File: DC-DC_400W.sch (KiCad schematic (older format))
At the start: 12 parts, among them J1 Conn_01x24, J2 Conn_01x03, J3 Conn_01x10, J4 Conn_01x10, J5 Conn_01x01, J6 Conn_01x02, J7 Conn_01x01, J8 Conn_01x01, J9 Conn_01x01

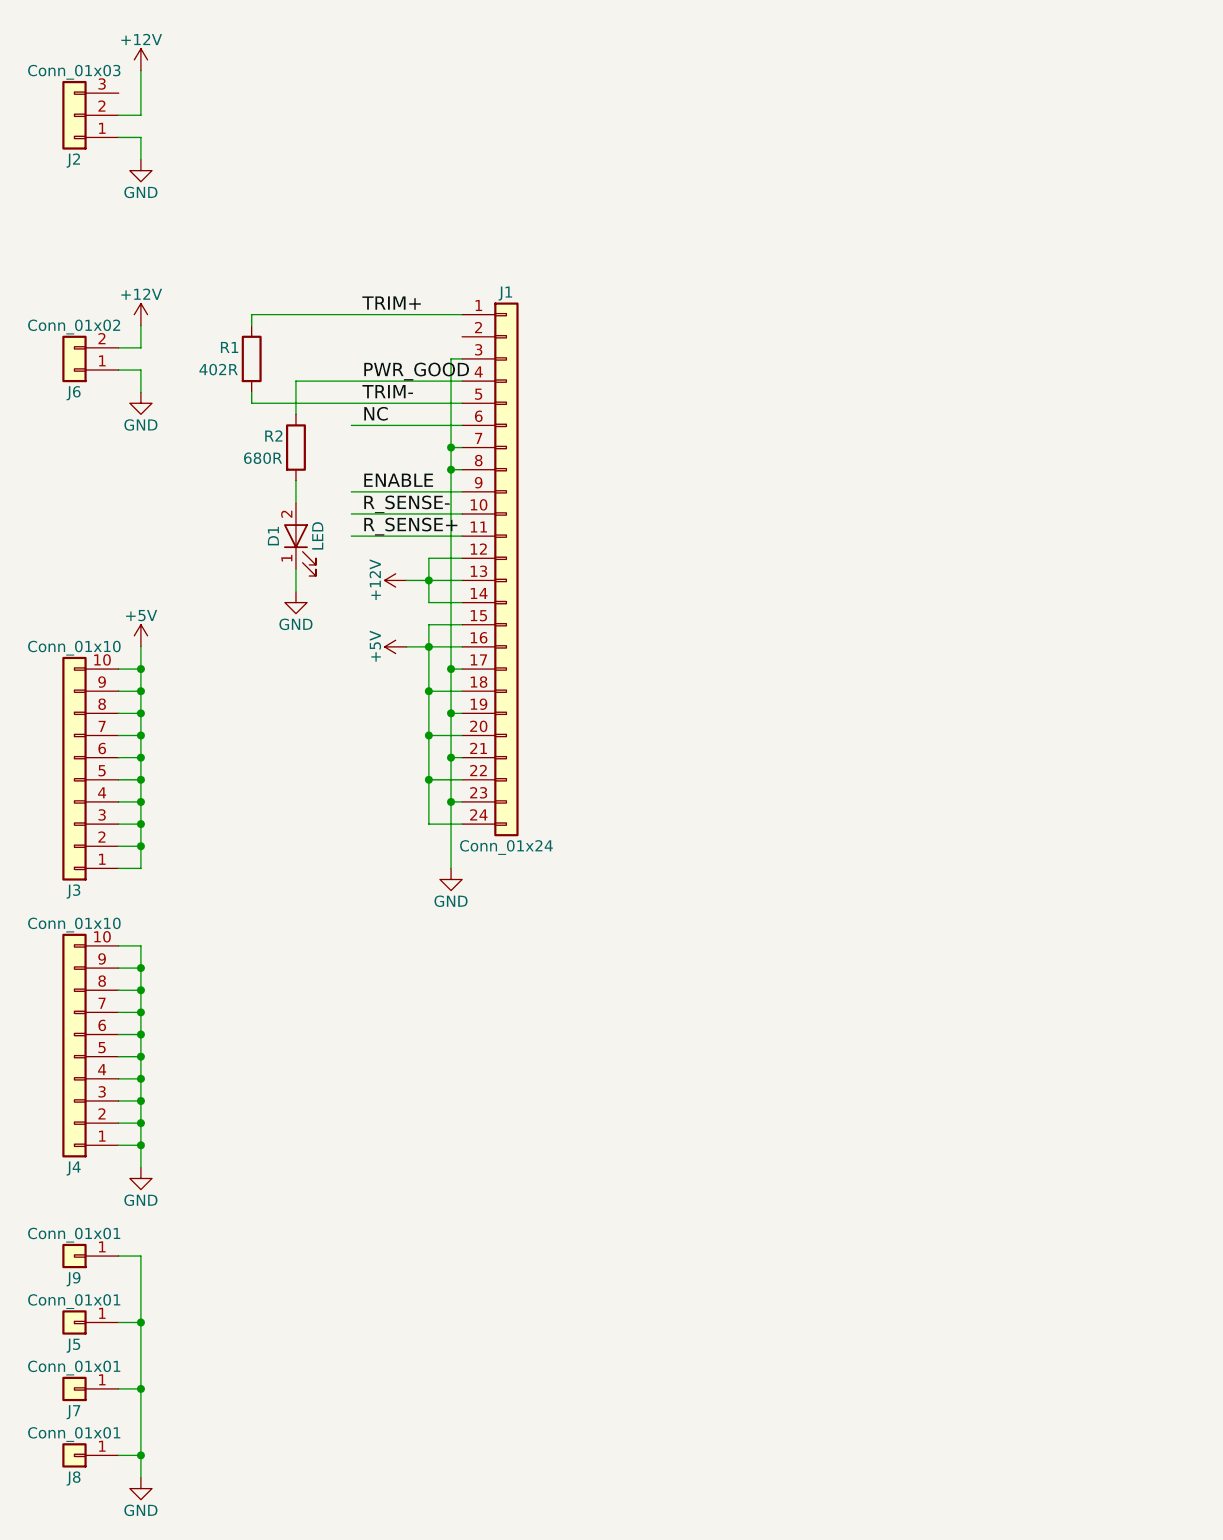
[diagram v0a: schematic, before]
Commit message: almost done
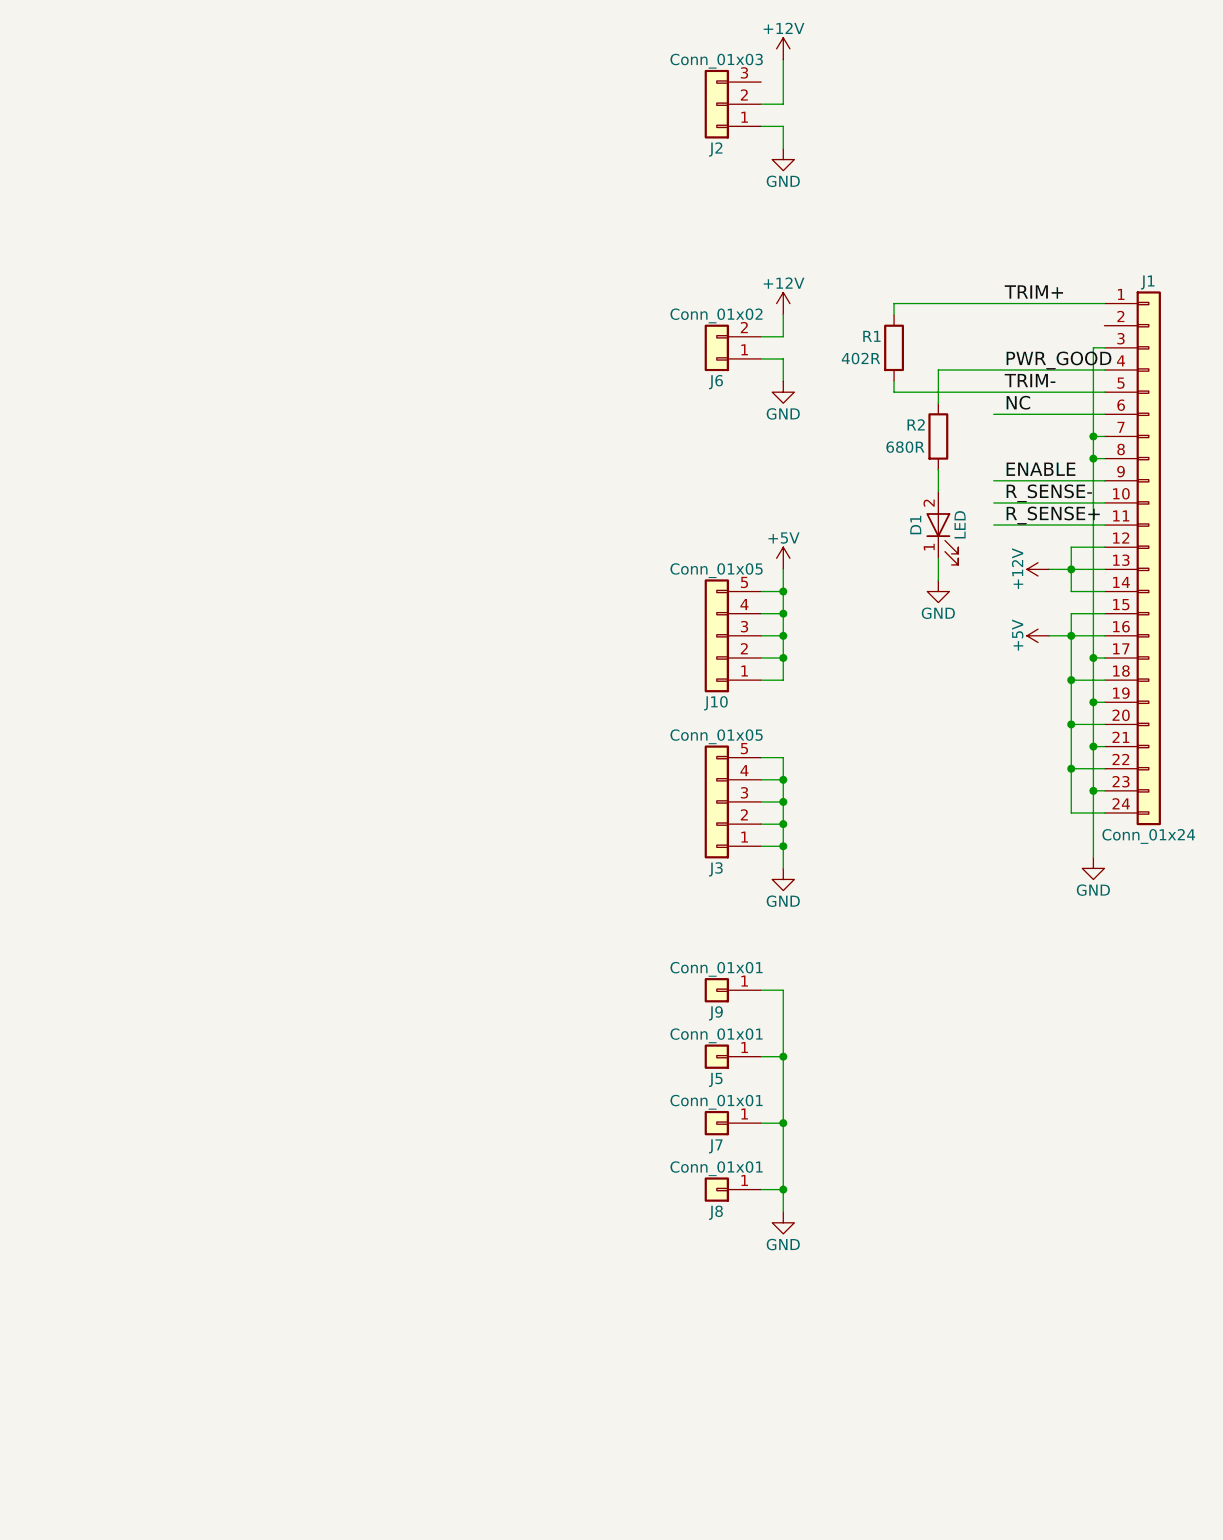
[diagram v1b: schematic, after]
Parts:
- removed J3, J4: Conn_01x10, Connectors_Phoenix:PhoenixContact_MSTBVA-G_10x5.00mm_Vertical, symbol Conn_01x10
- added J10, J3: Conn_01x05, Connectors_Phoenix:PhoenixContact_MSTBVA-G_05x5.00mm_Vertical, symbol Conn_01x05
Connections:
- wire segments 66 -> 56
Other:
- moved on the sheet: D1, J1, J2, J5, J6, J7, J8, J9, R1, R2
